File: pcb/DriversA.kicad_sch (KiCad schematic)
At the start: 49 parts, among them J13 54202-S0806ALF, J14 54202-S0806ALF, J5 TERM BLOCK, J6 TERM BLOCK, Q6 BSS84, Q7 BSS84, U3 TAS5720MRSMR, U4 TAS5720MRSMR

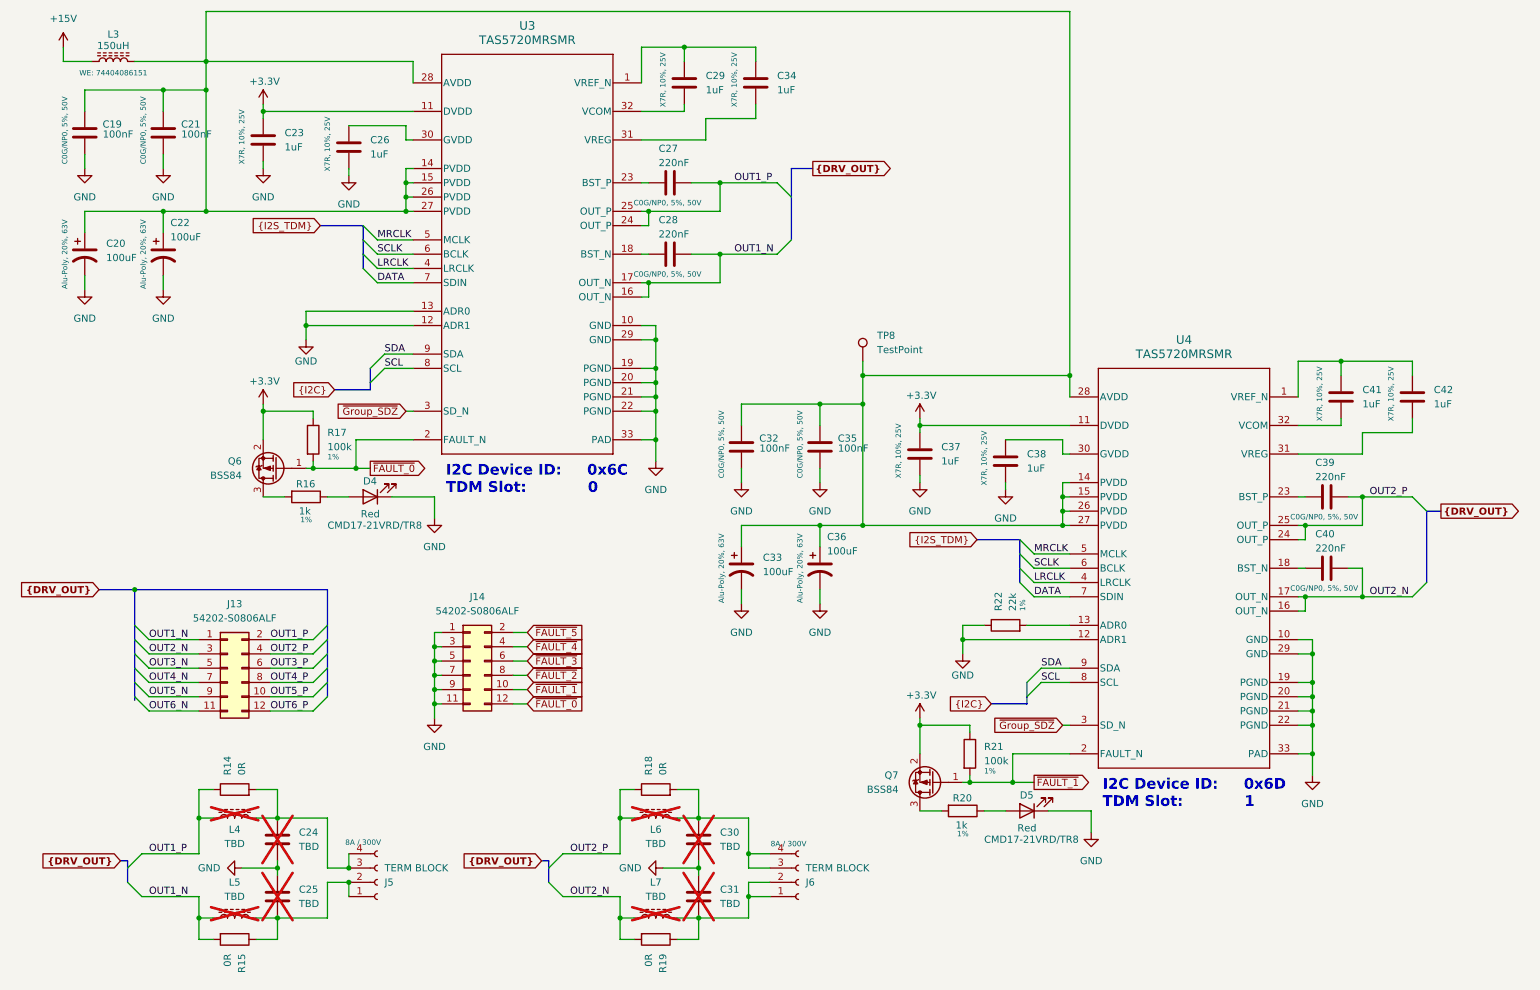
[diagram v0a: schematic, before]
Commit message: SIMULATED Transmission line, LAST checks, ORDERED pcb
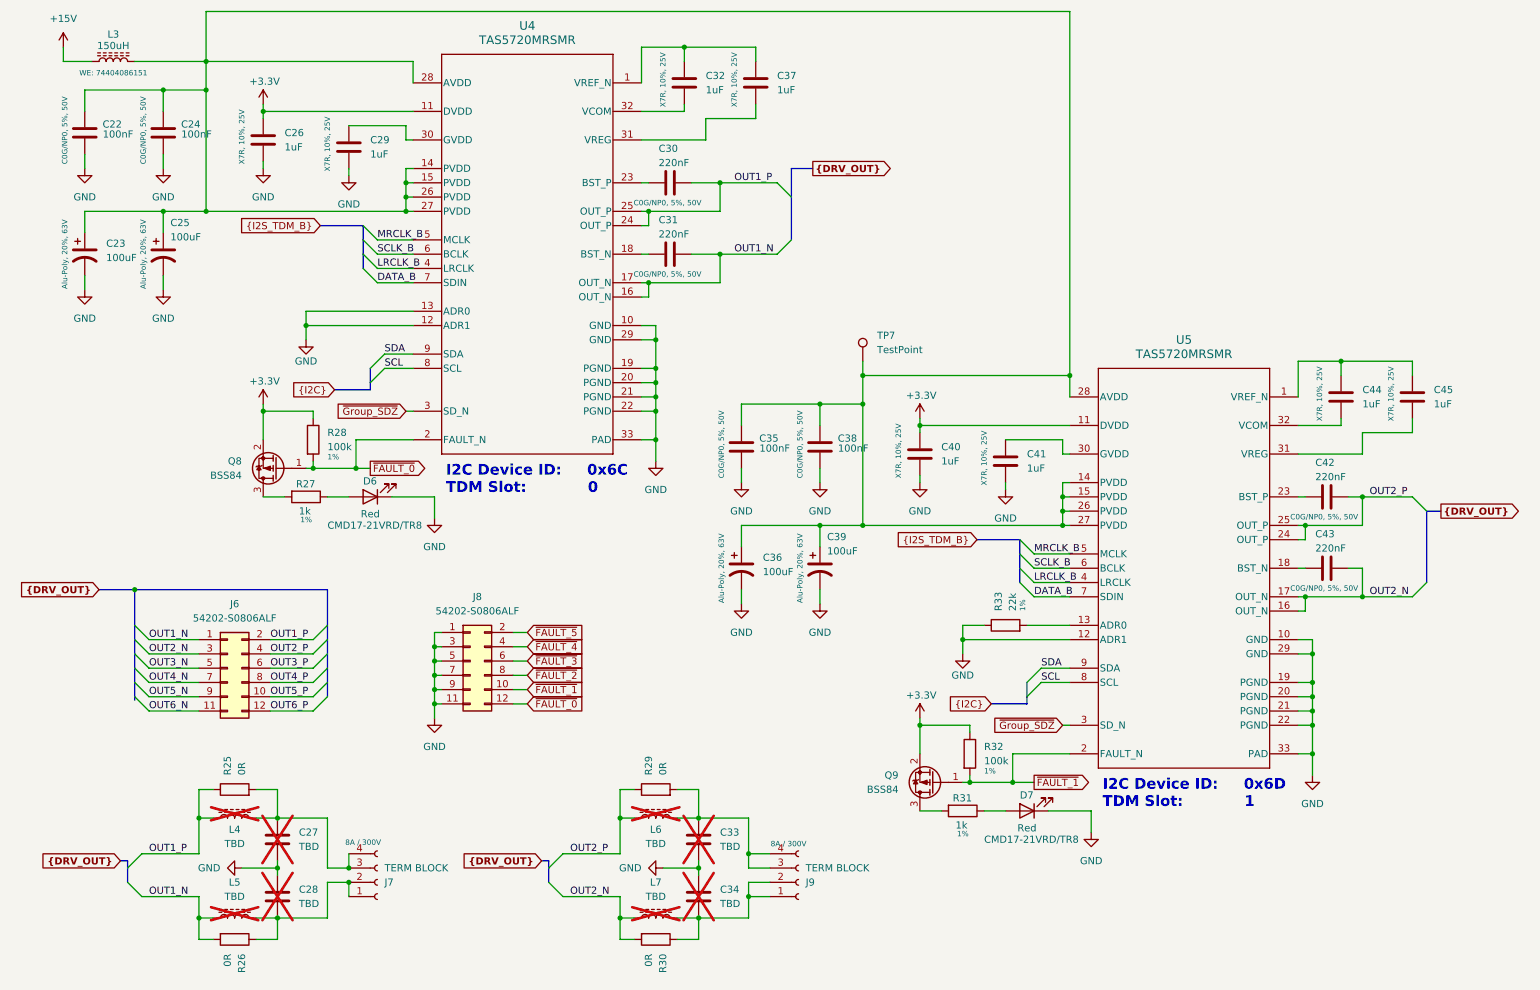
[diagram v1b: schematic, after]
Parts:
- renumbered C19 to C22, C20 to C23, C21 to C24, C22 to C25, C23 to C26, C24 to C27, C25 to C28, C26 to C29, C27 to C30, C28 to C31, C29 to C32, C30 to C33, C31 to C34, C32 to C35, C33 to C36, C34 to C37, C35 to C38, C36 to C39, C37 to C40, C38 to C41, C39 to C42, C40 to C43, C41 to C44, C42 to C45, D4 to D6, D5 to D7, J13 to J6, J5 to J7, J14 to J8, J6 to J9, Q6 to Q8, Q7 to Q9, R14 to R25, R15 to R26, R16 to R27, R17 to R28, R18 to R29, R19 to R30, R20 to R31, R21 to R32, R22 to R33, TP8 to TP7, U3 to U4, U4 to U5
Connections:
- net DATA renamed DATA_B
- net LRCLK renamed LRCLK_B
- net MRCLK renamed MRCLK_B
- net SCLK renamed SCLK_B
